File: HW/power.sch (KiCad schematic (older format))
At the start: 11 parts, among them J1 Vin, U1 LM2937, U2 LT1054

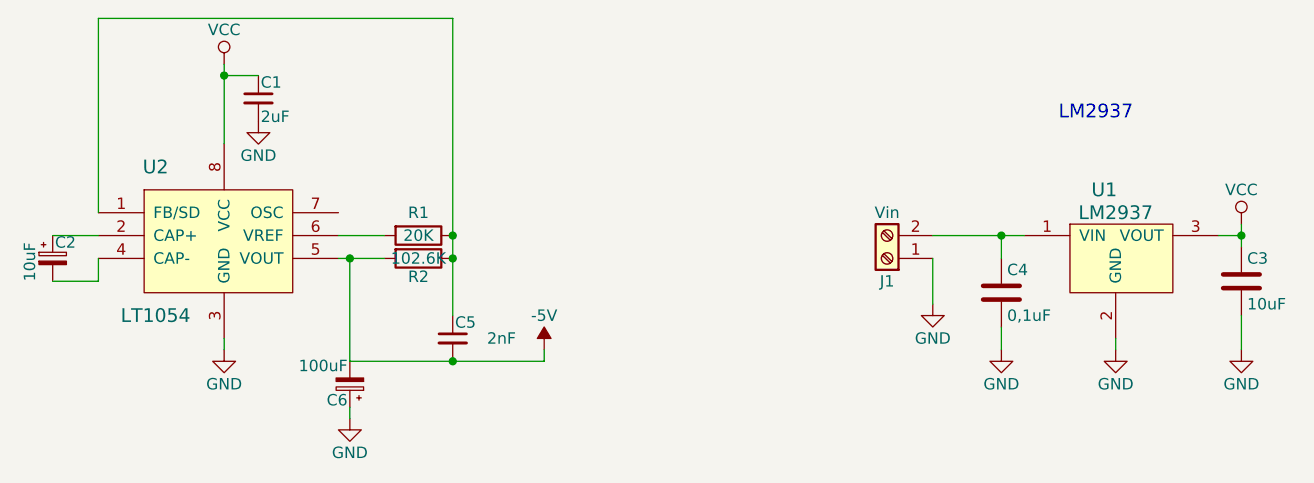
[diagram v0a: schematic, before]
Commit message: better layout
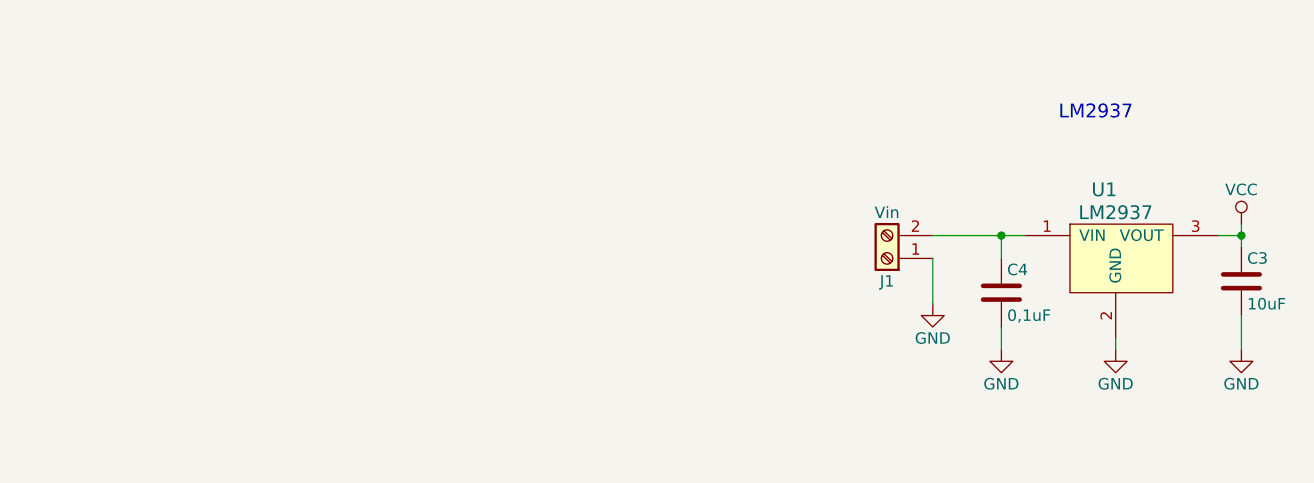
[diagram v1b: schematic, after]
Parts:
- removed C1: 2uF, Capacitors_SMD:C_0805_HandSoldering, symbol C_Small
- removed C2: 10uF, Capacitors_Tantalum_SMD:CP_Tantalum_Case-C_EIA-6032-28_Hand, symbol CP_Small
- removed C5: 2nF, Capacitors_SMD:C_0805_HandSoldering, symbol C_Small
- removed C6: 100uF, Capacitors_THT:CP_Radial_D6.3mm_P2.50mm, symbol CP_Small
- removed R1: 20K, Resistors_SMD:R_0805_HandSoldering, symbol R
- removed R2: 102.6K, Resistors_SMD:R_0805_HandSoldering, symbol R
- removed U2: LT1054, Housings_DIP:DIP-8_W7.62mm_LongPads, symbol LT1054
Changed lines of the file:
@@
 Comment4 ""
 $EndDescr
-$Comp
-L -5V #PWR6
-U 1 1 5A971C8A
-P 4050 3500
-F 0 "#PWR6" H 4050 3600 50  0001 C CNN
-F 1 "-5V" H 4050 3650 50  0000 C CNN
-F 2 "" H 4050 3500 50  0001 C CNN
-F 3 "" H 4050 3500 50  0001 C CNN
-	1    4050 3500
-	1    0    0    -1
-$EndComp
-$Comp
-L LT1054 U2
-U 1 1 5A971C9E
-P 2650 3200
-F 0 "U2" H 2350 3700 60  0000 C CNN
-F 1 "LT1054" H 2350 3050 60  0000 C CNN
-F 2 "Housings_DIP:DIP-8_W7.62mm_LongPads" H 2850 2750 60  0001 C CNN
-F 3 "http://www.ti.com/lit/ds/symlink/lt1054.pdf" H 3000 2850 60  0001 C CNN
-	1    2650 3200
-	1    0    0    -1
-$EndComp
-$Comp
-L GND #PWR01
-U 1 1 5A971D46
-P 2650 3500
-F 0 "#PWR01" H 2650 3250 50  0001 C CNN
-F 1 "GND" H 2650 3350 50  0000 C CNN
-F 2 "" H 2650 3500 50  0001 C CNN
-F 3 "" H 2650 3500 50  0001 C CNN
-	1    2650 3500
-	1    0    0    -1
-$EndComp
-Wire Wire Line
-	2650 3450 2650 3500
-$Comp
-L CP_Small C2
-U 1 1 5A971DAC
-P 1900 3100
-F 0 "C2" H 1910 3170 50  0000 L CNN
-F 1 "10uF" V 1800 3000 50  0000 L CNN
-F 2 "Capacitors_Tantalum_SMD:CP_Tantalum_Case-C_EIA-6032-28_Hand" H 1900 3100 50  0001 C CNN
-F 3 "" H 1900 3100 50  0001 C CNN
-	1    1900 3100
-	1    0    0    -1
-$EndComp
-Wire Wire Line
-	2100 3000 1900 3000
-Wire Wire Line
-	2100 3100 2100 3200
-Wire Wire Line
-	2100 3200 1900 3200
-$Comp
-L R R1
-U 1 1 5A971E49
-P 3500 3000
-F 0 "R1" V 3400 3000 50  0000 C CNN
-F 1 "20K" V 3500 3000 50  0000 C CNN
-F 2 "Resistors_SMD:R_0805_HandSoldering" V 3430 3000 50  0001 C CNN
-F 3 "" H 3500 3000 50  0001 C CNN
-	1    3500 3000
-	0    1    1    0
-$EndComp
-Wire Wire Line
-	3350 3000 3150 3000
-$Comp
-L VCC #PWR02
-U 1 1 5A971ED5
-P 2650 2250
-F 0 "#PWR02" H 2650 2100 50  0001 C CNN
-F 1 "VCC" H 2650 2400 50  0000 C CNN
-F 2 "" H 2650 2250 50  0001 C CNN
-F 3 "" H 2650 2250 50  0001 C CNN
-	1    2650 2250
-	1    0    0    -1
-$EndComp
-$Comp
-L C_Small C1
-U 1 1 5A971F06
-P 2800 2400
-F 0 "C1" H 2810 2470 50  0000 L CNN
-F 1 "2uF" H 2810 2320 50  0000 L CNN
-F 2 "Capacitors_SMD:C_0805_HandSoldering" H 2800 2400 50  0001 C CNN
-F 3 "" H 2800 2400 50  0001 C CNN
-	1    2800 2400
-	1    0    0    -1
-$EndComp
-$Comp
-L GND #PWR03
-U 1 1 5A971F51
-P 2800 2500
-F 0 "#PWR03" H 2800 2250 50  0001 C CNN
-F 1 "GND" H 2800 2350 50  0000 C CNN
-F 2 "" H 2800 2500 50  0001 C CNN
-F 3 "" H 2800 2500 50  0001 C CNN
-	1    2800 2500
-	1    0    0    -1
-$EndComp
-Wire Wire Line
-	2650 2250 2650 2600
-Wire Wire Line
-	2800 2300 2650 2300
-Connection ~ 2650 2300
-$Comp
-L R R2
-U 1 1 5A971FF1
-P 3500 3100
-F 0 "R2" V 3580 3100 50  0000 C CNN
-F 1 "102.6K" V 3500 3100 50  0000 C CNN
-F 2 "Resistors_SMD:R_0805_HandSoldering" V 3430 3100 50  0001 C CNN
-F 3 "" H 3500 3100 50  0001 C CNN
-	1    3500 3100
-	0    1    1    0
-$EndComp
-Wire Wire Line
-	3150 3100 3350 3100
-Wire Wire Line
-	2100 2900 2100 2050
-Wire Wire Line
-	2100 2050 3650 2050
-Wire Wire Line
-	3650 2050 3650 3350
-Connection ~ 3650 3000
-Wire Wire Line
-	3200 3100 3200 3550
-Wire Wire Line
-	3200 3550 4050 3550
-Connection ~ 3200 3100
-$Comp
-L CP_Small C6
-U 1 1 5A9720FC
-P 3200 3650
-F 0 "C6" H 3210 3720 50  0000 L CNN
-F 1 "100uF" H 3210 3570 50  0000 L CNN
-F 2 "Capacitors_THT:CP_Radial_D6.3mm_P2.50mm" H 3200 3650 50  0001 C CNN
-F 3 "" H 3200 3650 50  0001 C CNN
-	1    3200 3650
-	-1   0    0    1
-$EndComp
-$Comp
-L GND #PWR04
-U 1 1 5A972177
-P 3200 3800
-F 0 "#PWR04" H 3200 3550 50  0001 C CNN
-F 1 "GND" H 3200 3650 50  0000 C CNN
-F 2 "" H 3200 3800 50  0001 C CNN
-F 3 "" H 3200 3800 50  0001 C CNN
-	1    3200 3800
-	1    0    0    -1
-$EndComp
-Wire Wire Line
-	3200 3800 3200 3750
-Wire Wire Line
-	4050 3550 4050 3500
-Connection ~ 3650 3100
-$Comp
-L C_Small C5
-U 1 1 5A97221D
-P 3650 3450
-F 0 "C5" H 3660 3520 50  0000 L CNN
-F 1 "2nF" H 3800 3450 50  0000 L CNN
-F 2 "Capacitors_SMD:C_0805_HandSoldering" H 3650 3450 50  0001 C CNN
-F 3 "" H 3650 3450 50  0001 C CNN
-	1    3650 3450
-	1    0    0    -1
-$EndComp
-Connection ~ 3650 3550
 Text Notes 6300 2500 0    60   ~ 0
 LM2937
@@
 $EndComp
 $Comp
-L GND #PWR05
+L GND #PWR01
 U 1 1 5A9EEF79
 P 7100 3500
-F 0 "#PWR05" H 7100 3250 50  0001 C CNN
+F 0 "#PWR01" H 7100 3250 50  0001 C CNN
 F 1 "GND" H 7100 3350 50  0000 C CNN
 F 2 "" H 7100 3500 50  0001 C CNN
@@
 $EndComp
 $Comp
-L VCC #PWR06
+L VCC #PWR02
 U 1 1 5A9FDAE3
 P 7100 2950
-F 0 "#PWR06" H 7100 2800 50  0001 C CNN
+F 0 "#PWR02" H 7100 2800 50  0001 C CNN
 F 1 "VCC" H 7100 3100 50  0000 C CNN
 F 2 "" H 7100 2950 50  0001 C CNN
@@
 $EndComp
 $Comp
-L GND #PWR07
+L GND #PWR03
 U 1 1 5A9FDB9C
 P 6550 3500
-F 0 "#PWR07" H 6550 3250 50  0001 C CNN
+F 0 "#PWR03" H 6550 3250 50  0001 C CNN
 F 1 "GND" H 6550 3350 50  0000 C CNN
 F 2 "" H 6550 3500 50  0001 C CNN
@@
 $EndComp
 $Comp
-L GND #PWR08
+L GND #PWR04
 U 1 1 5A9FDBED
 P 6050 3500
-F 0 "#PWR08" H 6050 3250 50  0001 C CNN
+F 0 "#PWR04" H 6050 3250 50  0001 C CNN
 F 1 "GND" H 6050 3350 50  0000 C CNN
 F 2 "" H 6050 3500 50  0001 C CNN
@@
 Connection ~ 6050 3000
 $Comp
-L GND #PWR09
+L GND #PWR05
 U 1 1 5A9FDDD2
 P 5750 3300
-F 0 "#PWR09" H 5750 3050 50  0001 C CNN
+F 0 "#PWR05" H 5750 3050 50  0001 C CNN
 F 1 "GND" H 5750 3150 50  0000 C CNN
 F 2 "" H 5750 3300 50  0001 C CNN
